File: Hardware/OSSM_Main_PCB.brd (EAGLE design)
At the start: 114.3 x 45.4 mm, 10 parts, among them J1 PJ-037AH, U1 LOLIN32_PRODUCTION

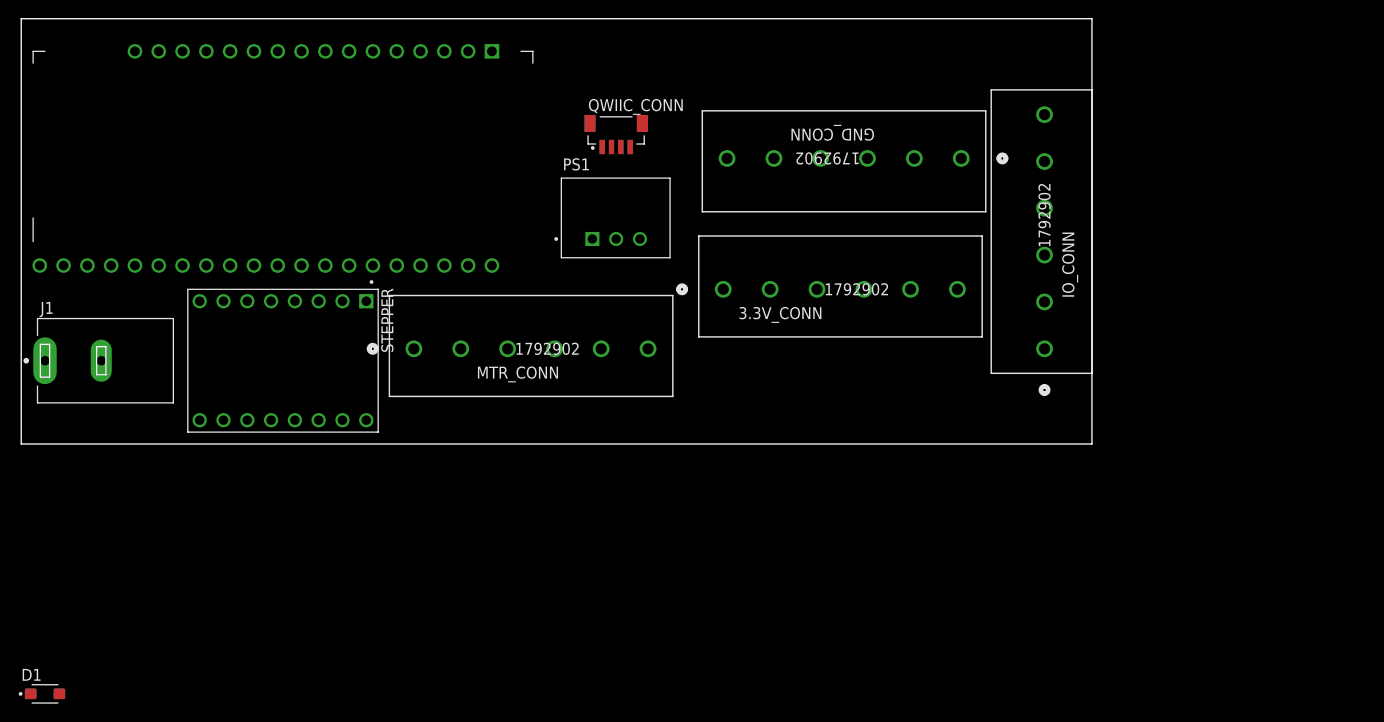
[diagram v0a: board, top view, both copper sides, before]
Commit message: James' Attempt
Maybe made it better, maybe made it worse?
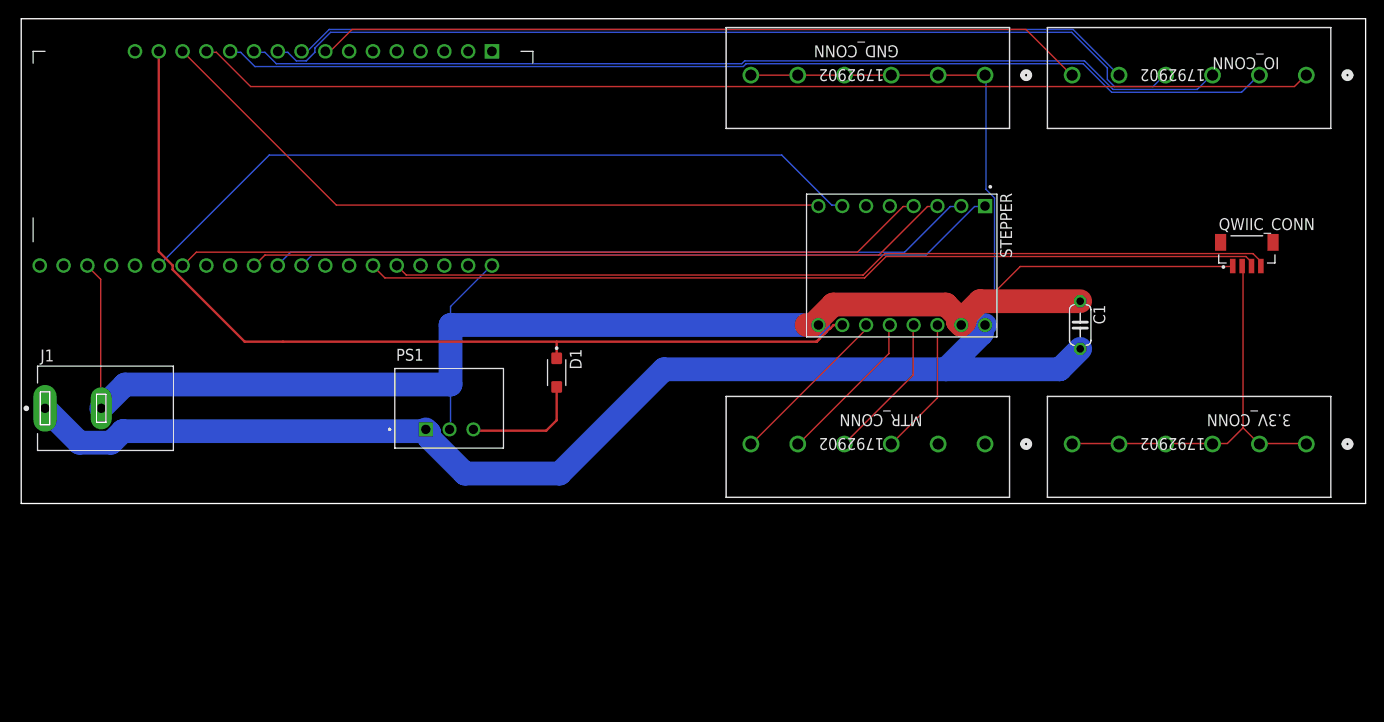
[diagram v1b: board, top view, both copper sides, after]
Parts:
- added C1: (no value), rcl:C050-024X044
- moved QWIIC_CONN 68.5 mm to (128.3, 53.3)
- moved STEPPER 66.8 mm to (91.4, 52.1)
- moved D1 64.5 mm to (54.6, 40.6), turned to 270 degrees
- moved 3.3V_CONN 64.4 mm to (134.6, 33.0), turned to 180 degrees
- moved MTR_CONN 61.8 mm to (100.3, 33.0), turned to 180 degrees
- moved IO_CONN 40.4 mm to (134.6, 72.4), turned to 180 degrees
- moved PS1 27.0 mm to (43.2, 36.8)
- moved GND_CONN 9.25 mm to (100.3, 72.4)
- moved J1 5.08 mm to (0.00, 36.8)
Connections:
- removed net VDD: STEPPER.10
- removed net VMOT: STEPPER.16
- new net N$10: MTR_CONN.4, STEPPER.13
- new net N$11: MTR_CONN.3, STEPPER.14
- new net N$12: IO_CONN.1, U1.13
- new net N$13: IO_CONN.2, U1.12
- new net N$14: IO_CONN.3, U1.11
- new net N$15: IO_CONN.4, U1.10
- new net N$16: IO_CONN.5, U1.9
- new net N$17: IO_CONN.6, U1.8
- new net N$2: STEPPER.1, U1.25
- new net N$3: STEPPER.2, U1.26
- new net N$4: STEPPER.3, U1.27
- new net N$5: STEPPER.4, U1.30
- new net N$6: STEPPER.7, U1.31
- new net N$7: STEPPER.8, U1.14
- new net N$8: MTR_CONN.6, STEPPER.11
- new net N$9: MTR_CONN.5, STEPPER.12
- net 24V: now also C1.2, STEPPER.16
- net 5V: now also STEPPER.10
- net GND: now also C1.1
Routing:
- net GND: track 0.00 -> 259.5 mm
- net 24V: track 0.00 -> 171.3 mm
- net 5V: track 0.00 -> 159.8 mm
- net N$12: track 0.00 -> 119.5 mm
- net N$13: track 0.00 -> 112.7 mm
- net N$14: track 0.00 -> 104.9 mm
- net N$15: track 0.00 -> 100.4 mm
- net 21_SDA: track 0.00 -> 96.0 mm
- net 22_SCL: track 0.00 -> 94.4 mm
- net N$16: track 0.00 -> 90.2 mm
- net N$17: track 0.00 -> 82.7 mm
- net N$5: track 0.00 -> 80.7 mm
- net N$6: track 0.00 -> 80.1 mm
- net N$4: track 0.00 -> 75.6 mm
- net N$3: track 0.00 -> 75.6 mm
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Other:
- board size 114.3 x 45.4 mm -> 143.5 x 51.7 mm
